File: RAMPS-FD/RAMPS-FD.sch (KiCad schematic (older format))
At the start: 17 parts, among them M101 LOGO_OSHW, P101 CONN_4, P102 VCC, P103 PS-ON, P104 5V, P105 12V-AUX, P106 CONN_3X2, SW101 SW_PUSH

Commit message: First version of RAMPS-FD, RIB
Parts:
- removed P101: CONN_4, symbol CONN_4
- added F103: FUSE 10A, symbol FUSE
- added J101, J103: NET-TIE, TIE-1MM, symbol NET-TIE
- added JP101: VSEL, symbol JUMP_MINI_3
- added P101: HB_IN, symbol CONN_2
- added P107: MOT_IN, symbol CONN_2
- added P108: POWER_IN, symbol CONN_2
- F101: value MFR1100 -> FUSE 15A
- F102: value MFR500 -> FUSE 10A
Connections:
- net labels added: +V_HEATBED, +V_LOGIC, +V_MOTOR, +V_POWER, /ESTOP, A6, A7, D51, E2_DIR, E2_EN, E2_STEP, FET4, GNDPWR, HB_GND, HB_IN, MOT_GND, MOT_IN, P_IN, SERVO1, SERVO2, SERVO3, SERVO4, THERM3, UART_RX_LVC, UART_TX_LVC, VCC
- net labels removed: +12P, +12V, A10, A11, A12, A3, A9, D11, D12, D16, D17, D32, D4, D40, D42, D44, D5, D6, SER1, SER2, SER3, SER4, UART_RX, UART_TX
- wire segments 133 -> 150
- no-connect marks 10 -> 11
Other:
- note added: "5V standby?"
- note added: "Extruder heaters, fans,\nDue/Mega input\n9-15V"
- note added: "Heatbed Only: 12-24V, 15A"
- note added: "Motors only, 12-24V"
- note added: "Note: On R3 compatible Arduinos, IOREF \nwill supply 3.3V (Due), or 5V (Mega).\n\nIf IOREF is not provided (non-R3) then it \nmust be a 5V Arduino so set VSEL to 5V.\n\nIf not 5V then need to get 3.3V from somewhere ..."
- note added: "VSEL - Select logic voltage\n1-2 = Autoselect by IOREF\n2-3 = 5V"
- note added: "X/Y/Z pins \non one port"
- moved on the sheet: C101, C102, D101, D102, D103, F101, F102, M101, P102, P103, P104, P105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

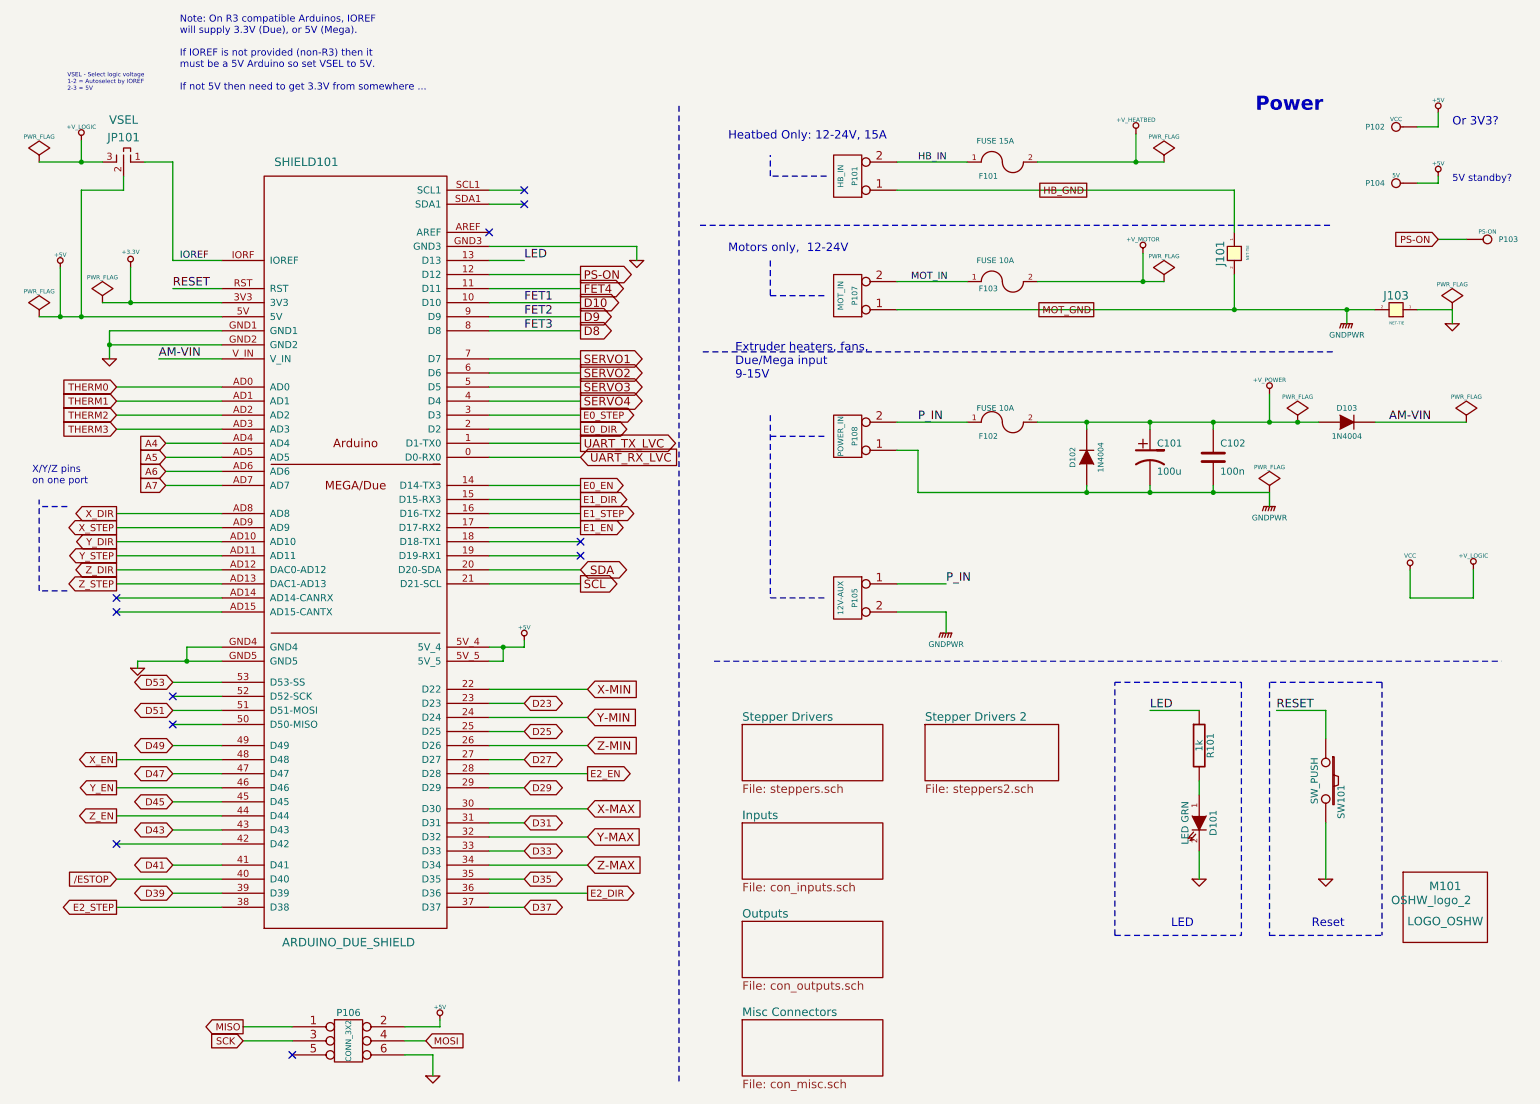
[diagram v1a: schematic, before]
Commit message: RAMPS-FD update
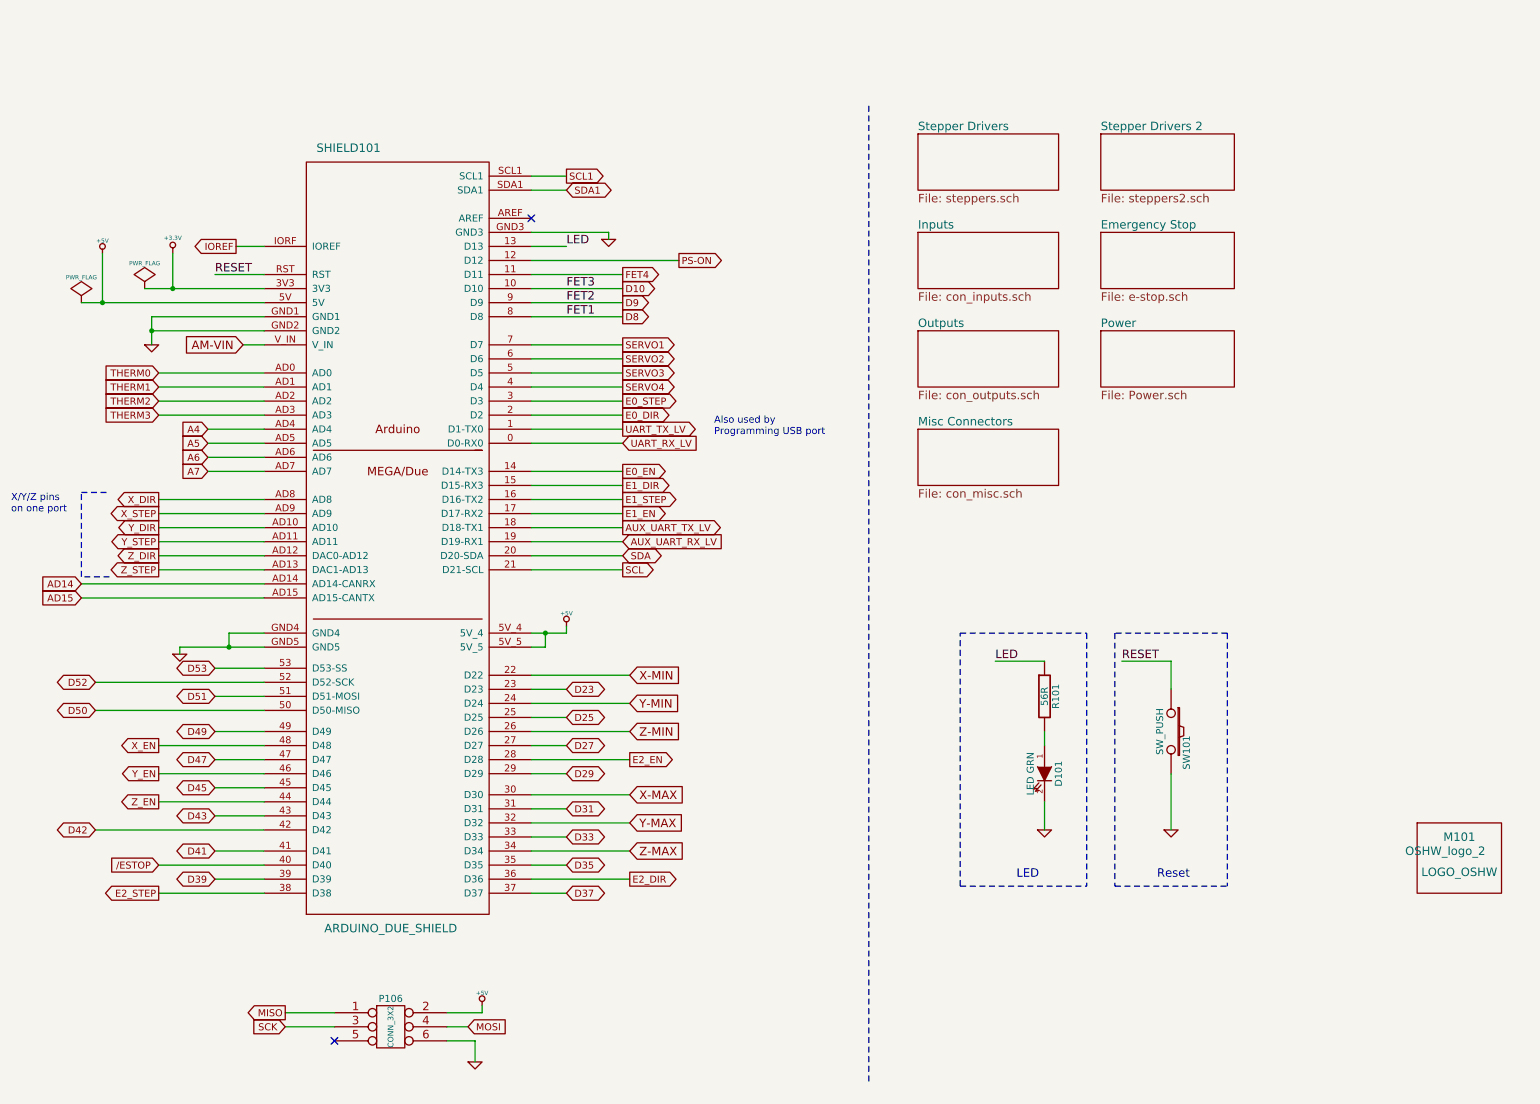
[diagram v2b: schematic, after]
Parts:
- removed C101: 100u, symbol CP1
- removed C102: 100n, symbol C
- removed D102, D103: 1N4004, symbol DIODE
- removed F101: FUSE 15A, symbol FUSE
- removed F102, F103: FUSE 10A, symbol FUSE
- removed J101, J103: NET-TIE, TIE-1MM, symbol NET-TIE
- removed JP101: VSEL, symbol JUMP_MINI_3
- removed P101: HB_IN, symbol CONN_2
- removed P102: VCC, symbol CONN_1
- removed P103: PS-ON, symbol CONN_1
- removed P104: 5V, symbol CONN_1
- removed P105: 12V-AUX, symbol CONN_2
- removed P107: MOT_IN, symbol CONN_2
- removed P108: POWER_IN, symbol CONN_2
- R101: value 1k -> 56R
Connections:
- net AUX_UART_TX_LV: now reaches SHIELD101.18 (D18-TX1)
- net AUX_UART_RX_LV: now reaches SHIELD101.19 (D19-RX1)
- net D42: now reaches SHIELD101.42 (D42)
- net D50: now reaches SHIELD101.50 (D50-MISO)
- net D52: now reaches SHIELD101.52 (D52-SCK)
- net AD14: now reaches SHIELD101.AD14 (AD14-CANRX)
- net AD15: now reaches SHIELD101.AD15 (AD15-CANTX)
- net SCL1: now reaches SHIELD101.SCL1
- net SDA1: now reaches SHIELD101.SDA1
- net UART_RX_LVC renamed UART_RX_LV
- net UART_TX_LVC renamed UART_TX_LV
- no-connect marks 11 -> 2
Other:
- note added: "Also used by\nProgramming USB port"
- note removed: "5V standby?"
- note removed: "Extruder heaters, fans,\nDue/Mega input\n9-15V"
- note removed: "Heatbed Only: 12-24V, 15A"
- note removed: "Motors only, 12-24V"
- note removed: "Note: On R3 compatible Arduinos, IOREF \nwill supply 3.3V (Due), or 5V (Mega).\n\nIf IOREF is not provided (non-R3) then it \nmust be a 5V Arduino so set VSEL to 5V.\n\nIf not 5V then need to get 3.3V from somewhere ..."
- note removed: "Or 3V3?"
- note removed: "Power"
- note removed: "VSEL - Select logic voltage\n1-2 = Autoselect by IOREF\n2-3 = 5V"
- moved on the sheet: D101, M101, P106, R101, SHIELD101, SW101
